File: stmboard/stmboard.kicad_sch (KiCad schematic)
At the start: 80 parts, among them J1 USB_C_Receptacle_USB2.0_14P, J2 Conn_02x05_Odd_Even, J3 USB_C_Receptacle_USB2.0_14P, J4 Conn_01x20_Socket, J5 Conn_01x20_Socket, J6 USB_C_Receptacle_USB2.0_14P, J7 Micro_SD_Card, J8 Conn_01x04, SW1 BOOT0, SW2 NRST, SW3 BOOT, SW4 BOOT, U1 STM32F411RCTx, U10 MAX98357A, U2 ESP32-S3-WROOM-1, U3 AP2112K-3.3, U4 AP2112K-3.3, U5 CP2102N-Axx-xQFN20, U6 AP2112K-3.3, U7 ICM-20948, U8 TXB0102DCT, U9 AP2112K-1.8, Y1 25MHz, Y2 32.768KHz

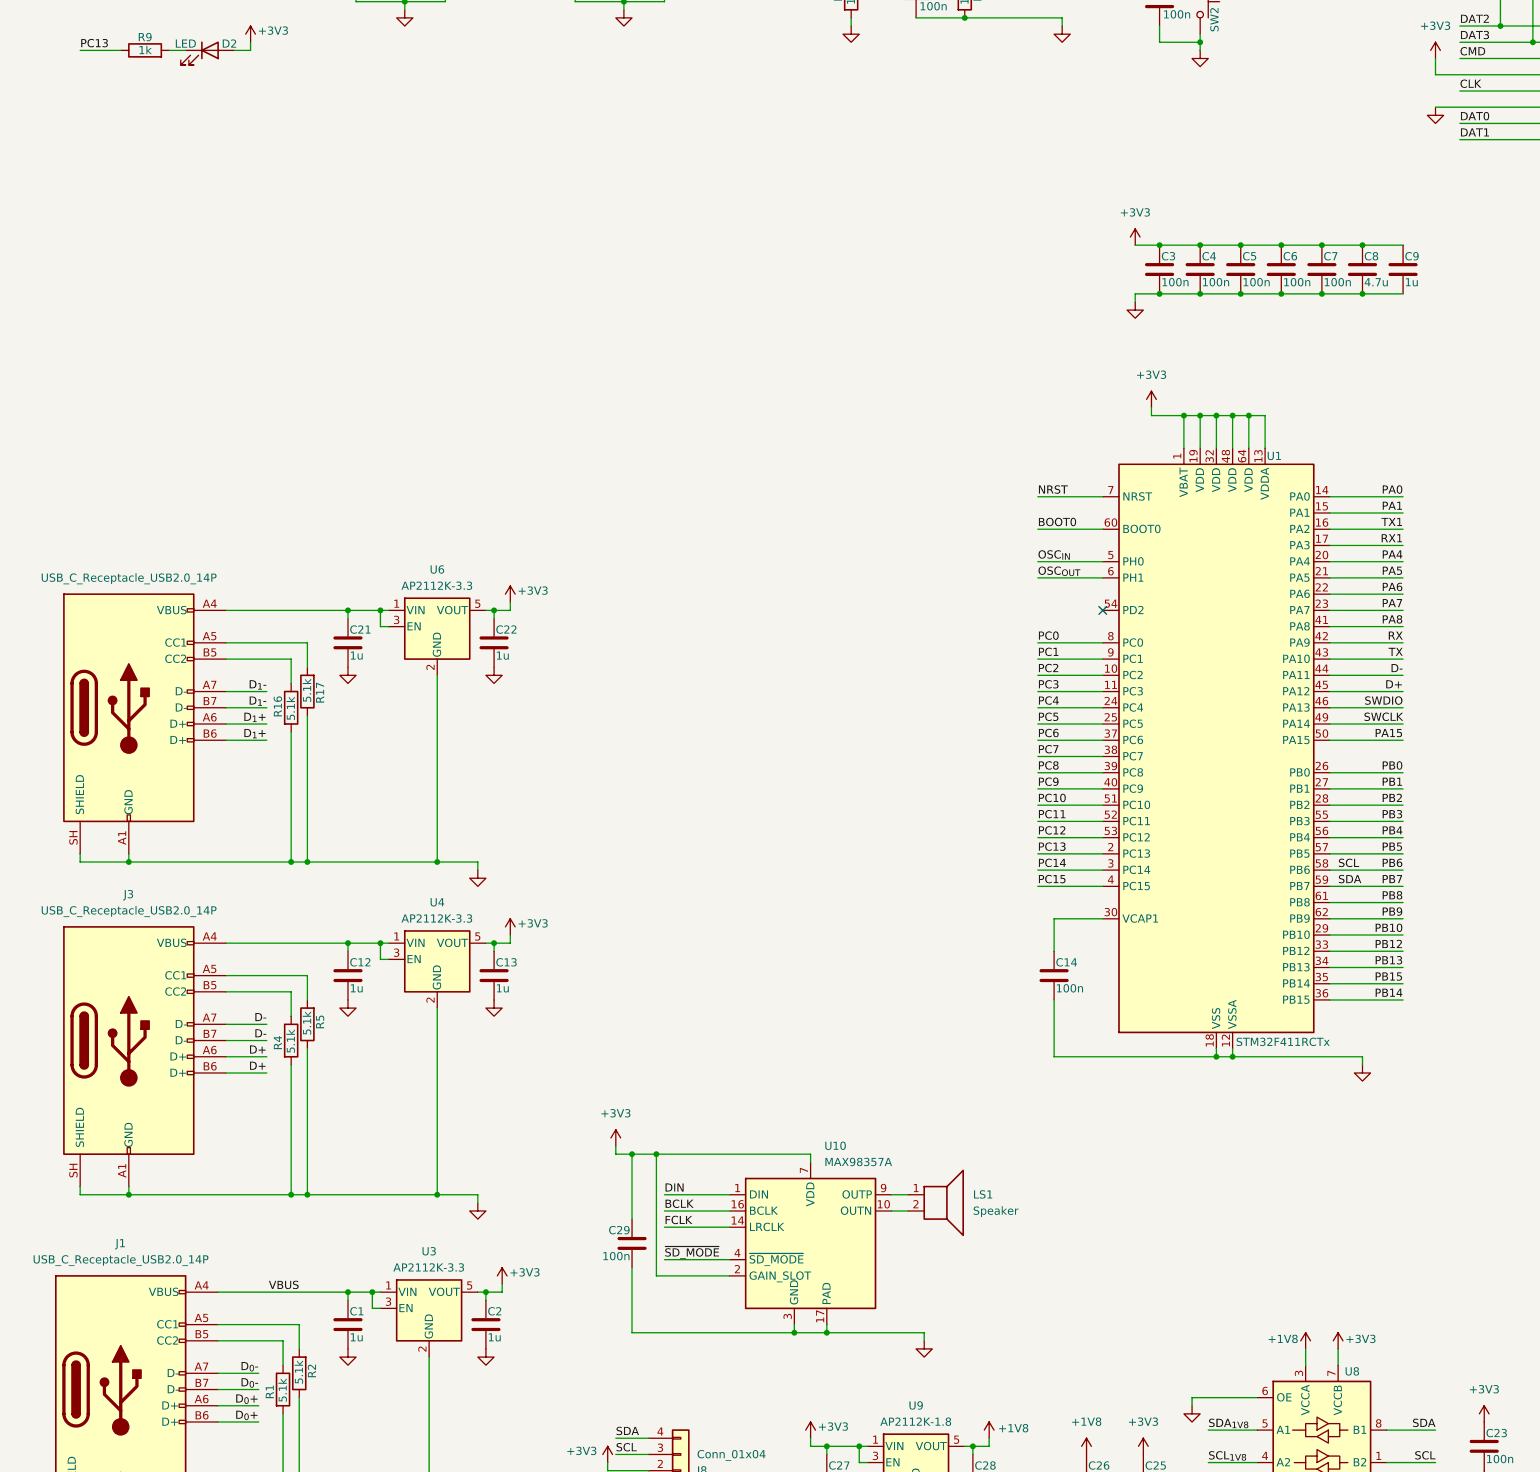
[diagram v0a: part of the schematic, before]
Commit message: mic + footprints
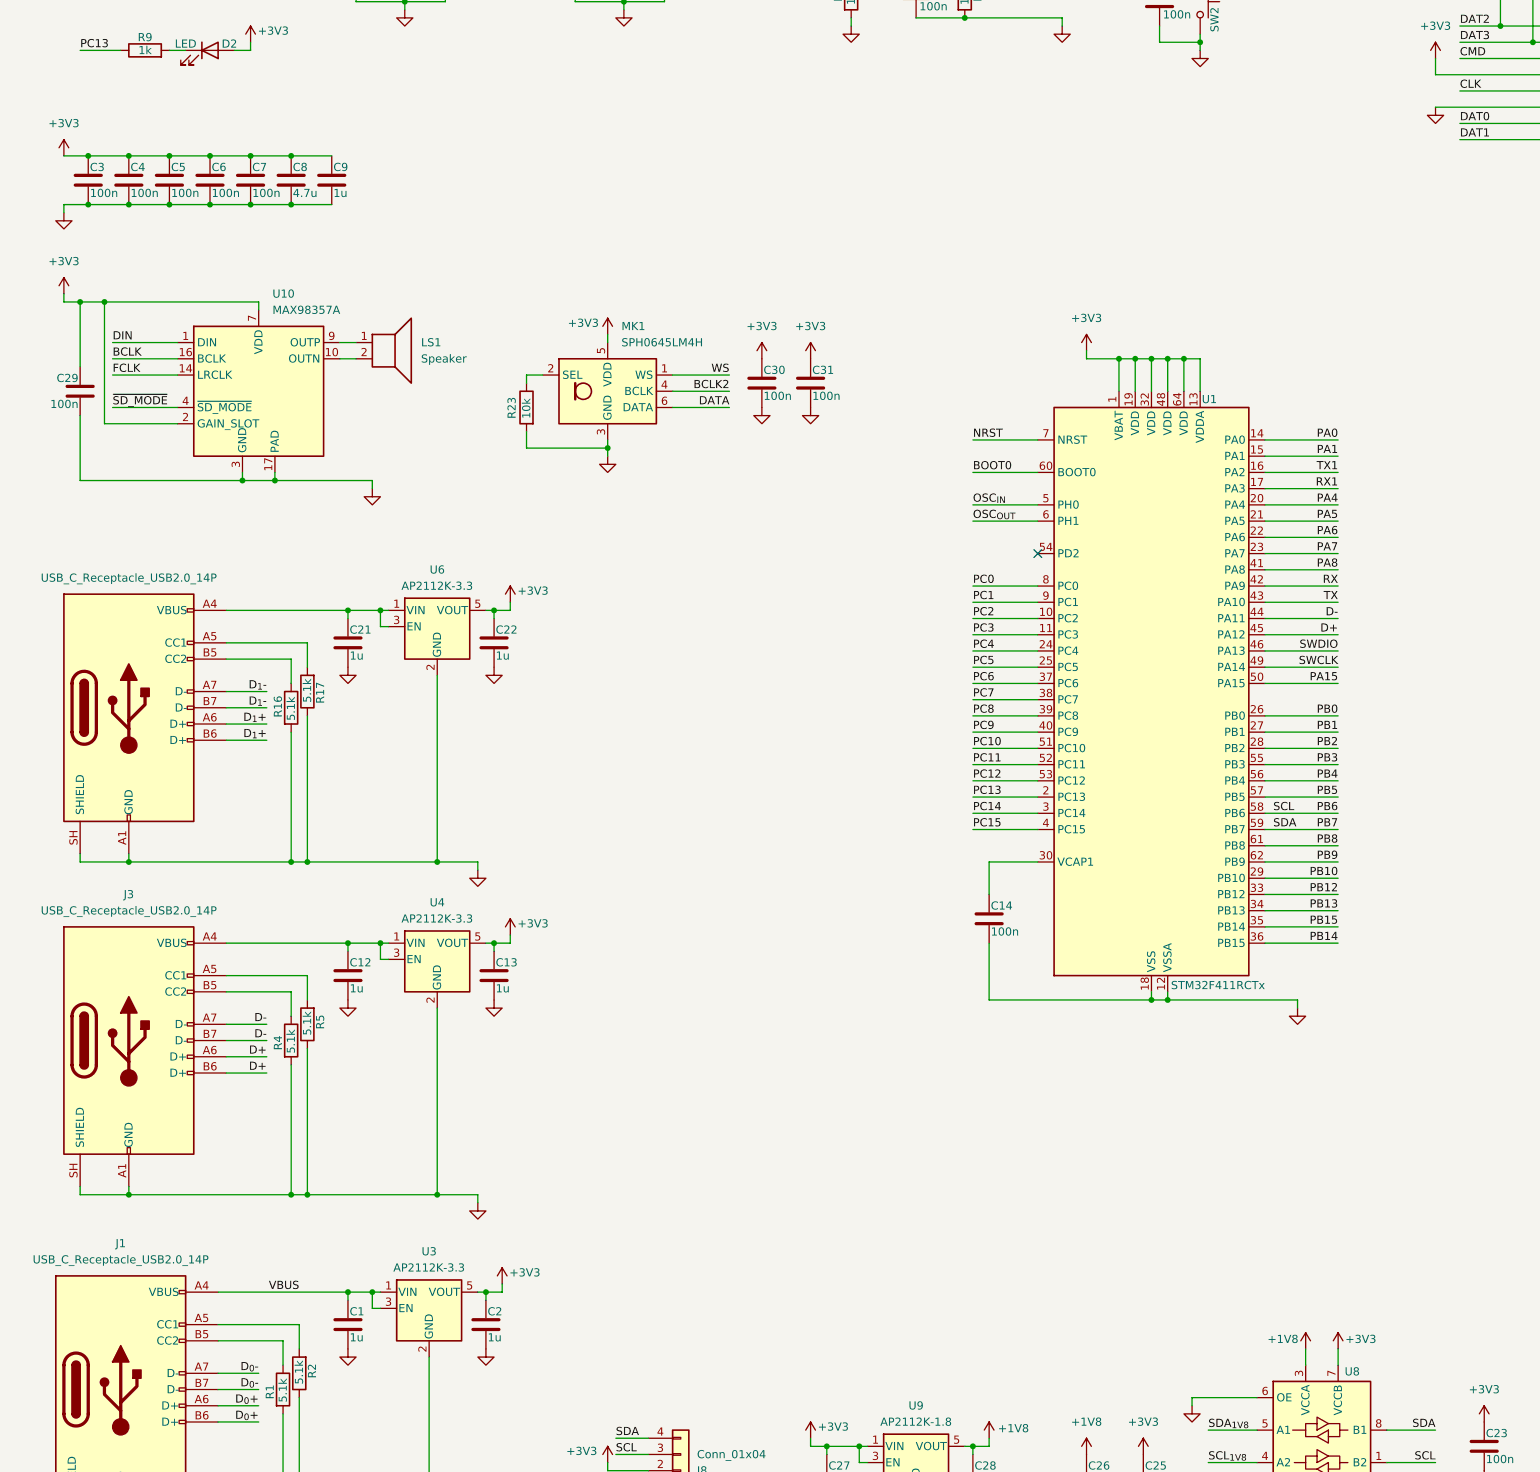
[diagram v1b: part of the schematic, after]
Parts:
- added C30, C31: 100n, Capacitor_SMD:C_0603_1608Metric, symbol Device:C
- added MK1: SPH0645LM4H, Sensor_Audio:Knowles_SPH0645LM4H-6_3.5x2.65mm, symbol Sensor_Audio:SPH0645LM4H
- added R23: 10k, symbol Device:R
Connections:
- net +3V3: now also C30.1, C31.1, MK1.5 (VDD)
- net GND: now also C30.2, C31.2, MK1.3 (GND), R23.2
- new net: MK1.2 (SEL), R23.1
- new net BCLK2: MK1.4 (BCLK)
- new net DATA: MK1.6 (DATA)
- new net WS: MK1.1 (WS)
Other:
- moved on the sheet: C14, C29, C3, C4, C5, C6, C7, C8, C9, LS1, U1, U10
